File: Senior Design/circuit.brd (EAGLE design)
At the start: 52 x 84.8 mm, 25 parts, among them IC1 74HC164N, IC2 ATMEGA328P, IC3 ATTINY24A, Q1 16 MHz

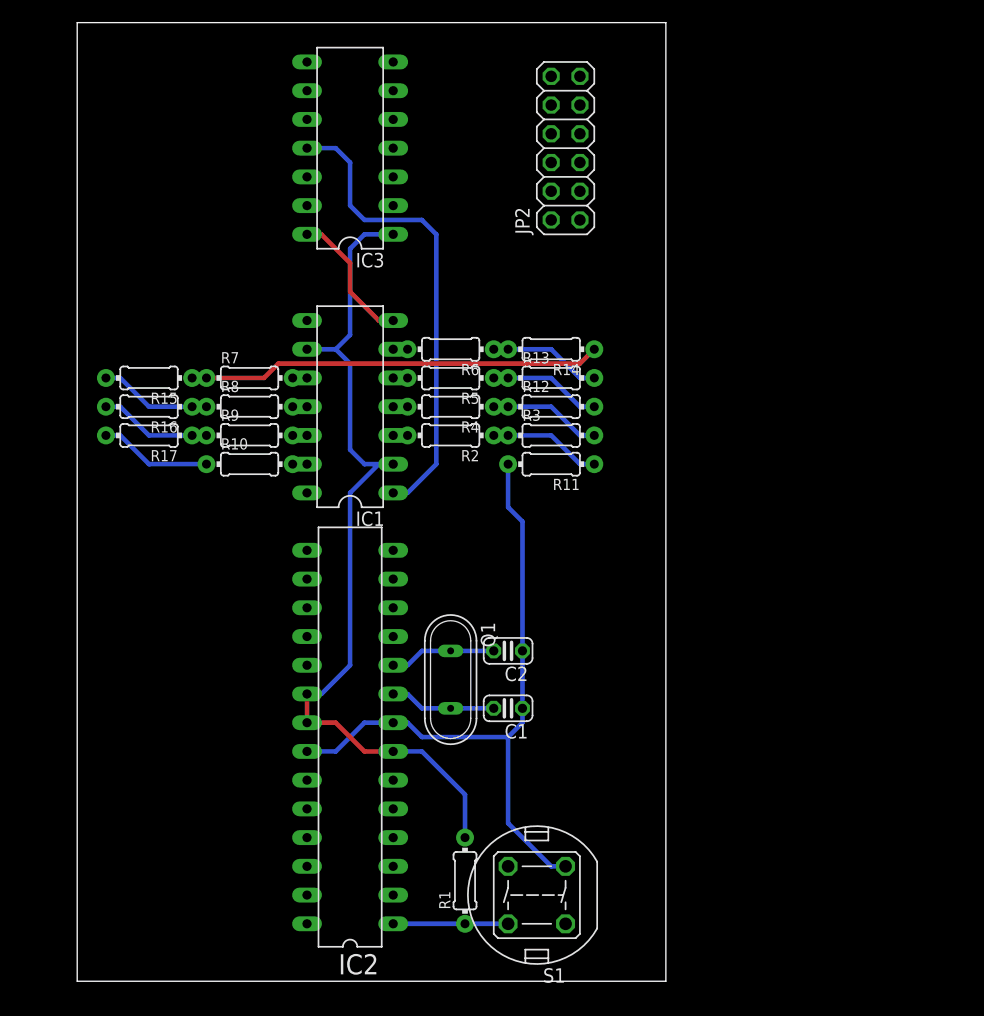
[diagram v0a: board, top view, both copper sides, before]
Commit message: working on senior design circuit and pcb
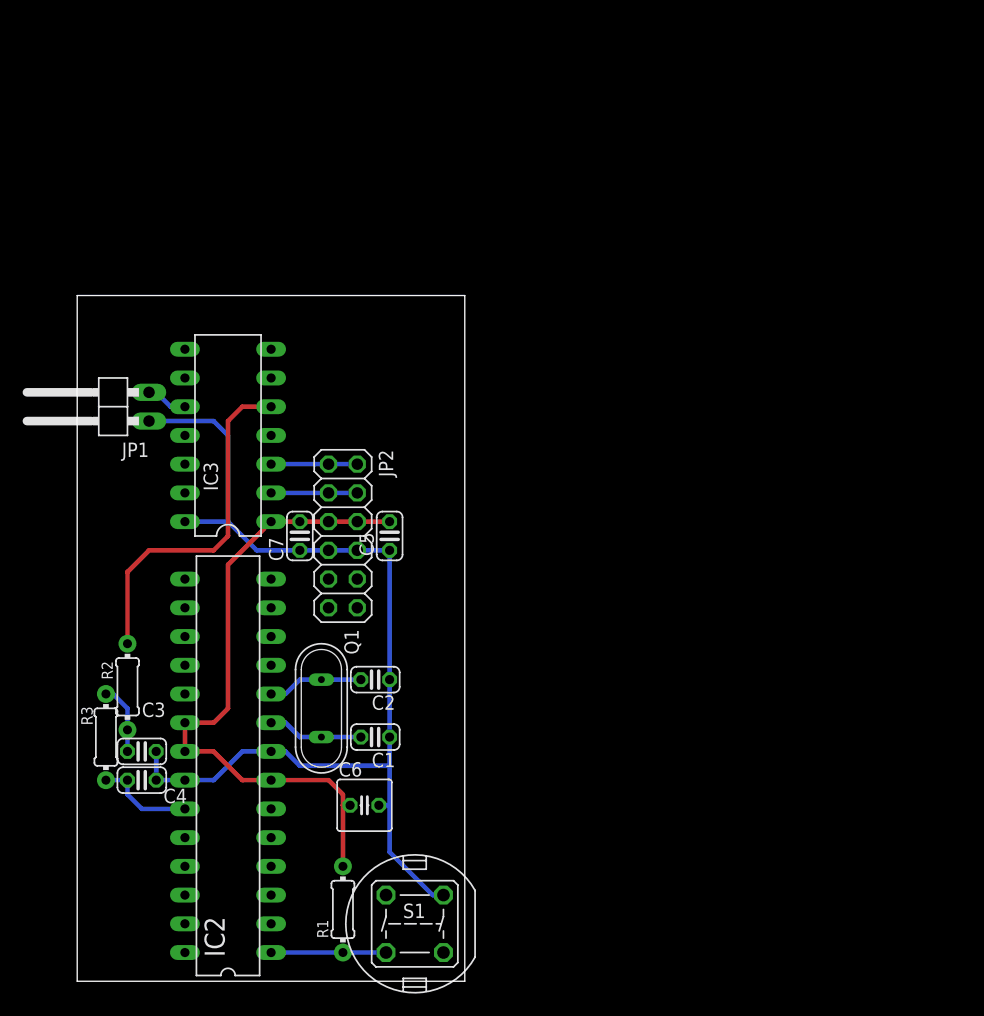
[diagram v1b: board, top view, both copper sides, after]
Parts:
- removed IC1: 74HC164N, 74xx-us:DIL14
- removed R10, R11, R4, R5, R6, R7, R8, R9: 10 kΩ, resistor:0204/7
- removed R12, R13, R14, R15, R16, R17: 4.7 kΩ, resistor:0204/7
- added C3, C4, C5, C7: 10nf, rcl:C025-024X044
- added C6: 100uF, rcl:C025-050X050
- added JP1: (no value), pinhead:1X02/90
- Q1: value 16 MHz -> 16MHz
- R3: value 4.7 kΩ -> 10 kΩ
- moved R3 47.6 mm to (2.54, 21.6), turned to 90 degrees
- moved JP2 39.5 mm to (23.5, 39.4), turned to 270 degrees
- moved R2 36.2 mm to (4.45, 26.0), turned to 90 degrees
- moved IC3 27.6 mm to (12.1, 41.9)
- moved C1 12.0 mm to (26.4, 21.6)
- moved C2 12.0 mm to (26.4, 26.7)
- moved Q1 11.7 mm to (21.6, 24.1)
- moved S1 11.1 mm to (29.8, 5.08)
- moved IC2 11.1 mm to (13.3, 19.1)
- moved R1 11.1 mm to (23.5, 6.35)
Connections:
- removed net N$10: R11.1, R2.1, R3.1
- removed net N$11: R14.1, R15.1, R7.1
- removed net N$12: R15.2, R16.1, R8.1
- removed net N$13: R16.2, R17.1, R9.1
- removed net N$14: R12.2, R13.1, R5.1
- removed net N$15: R12.1, R3.2, R4.1
- removed net N$17: R10.1, R17.2
- removed net N$19: IC1.11, R8.2
- removed net N$25: IC1.4, R4.2
- removed net N$26: IC1.5, R5.2
- removed net N$27: IC1.6, R6.2
- removed net N$28: IC1.10, R7.2
- removed net N$30: IC1.12, R9.2
- removed net N$31: IC1.13, R10.2
- removed net VCC: IC1.14
- net +5V: now also C5.2, C6.1, C7.2, JP2.5, JP2.6; no longer IC1.2, IC1.9, JP2.1, JP2.3
- net GND: now also C3.1, C4.1, C5.1, C6.2, C7.1, JP1.1, JP2.8; no longer IC1.7, JP2.5, R11.2, S1.3
- net N$1: now also IC3.2, JP2.3; no longer IC3.3
- net N$2: now also IC3.3, JP2.1; no longer IC3.2
- net N$3: now also IC3.10, JP1.2; no longer IC1.8, IC3.12
- net N$4: now also IC3.5, R2.2; no longer IC1.1, IC3.11
- net N$7: now also C3.2, R2.1, R3.2; no longer R13.2, R14.2, R6.1
- net N$8: no longer S1.1
- net N$9: now also C4.2, IC2.23, R3.1; no longer IC1.3, R2.2
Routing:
- net N$11: track 36.6 -> 0.00 mm
- net GND: track 71.1 -> 93.0 mm
- net +5V: track 76.7 -> 58.0 mm
- net N$4: track 42.0 -> 31.1 mm
- net N$14: track 9.94 -> 0.00 mm
- net N$12: track 9.94 -> 0.00 mm
- net N$17: track 9.94 -> 0.00 mm
- net N$15: track 9.94 -> 0.00 mm
- net N$13: track 9.94 -> 0.00 mm
- net N$10: track 9.94 -> 0.00 mm
- net N$2: track 0.00 -> 7.62 mm
- net N$1: track 0.00 -> 7.62 mm
- net N$9: track 1.27 -> 8.78 mm
- net N$7: track 11.2 -> 6.24 mm
- net N$3: track 0.00 -> 3.70 mm
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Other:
- board size 52 x 84.8 mm -> 34.3 x 60.6 mm

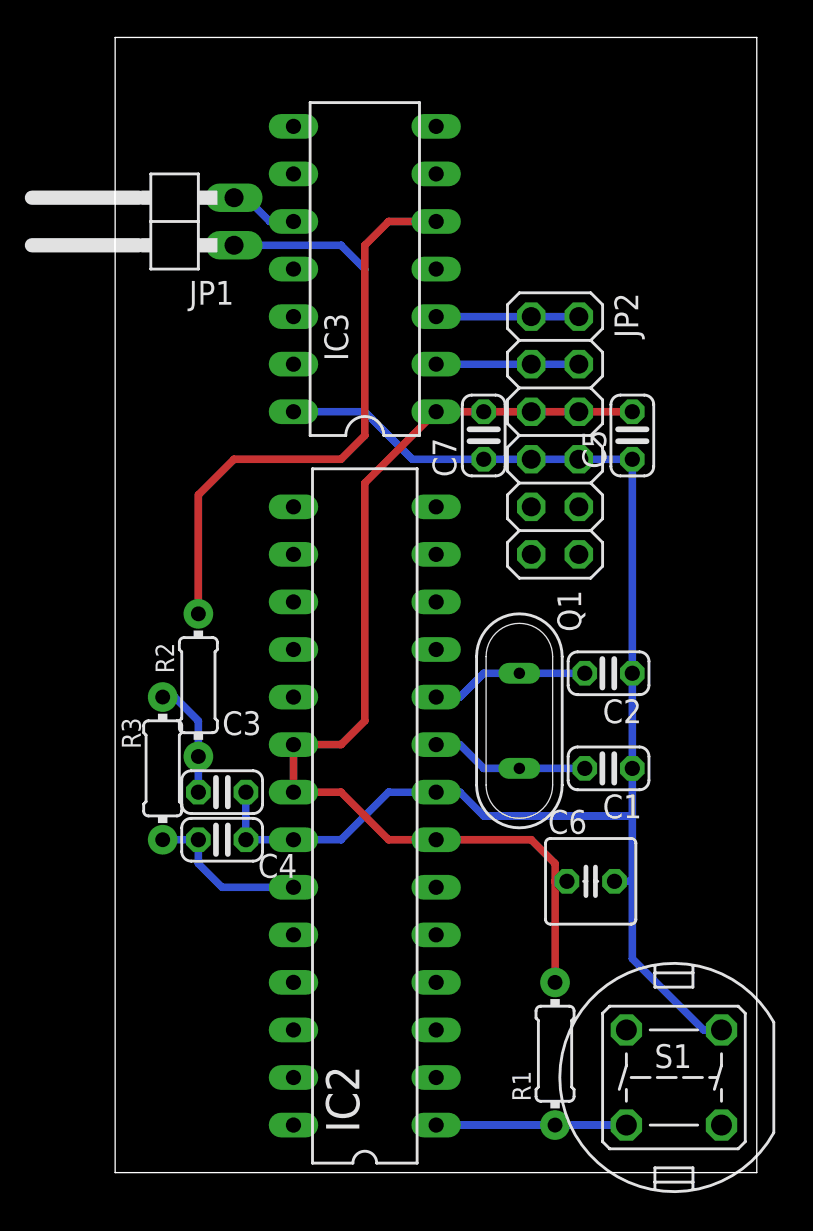
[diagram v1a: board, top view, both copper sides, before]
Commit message: worked on the schematic
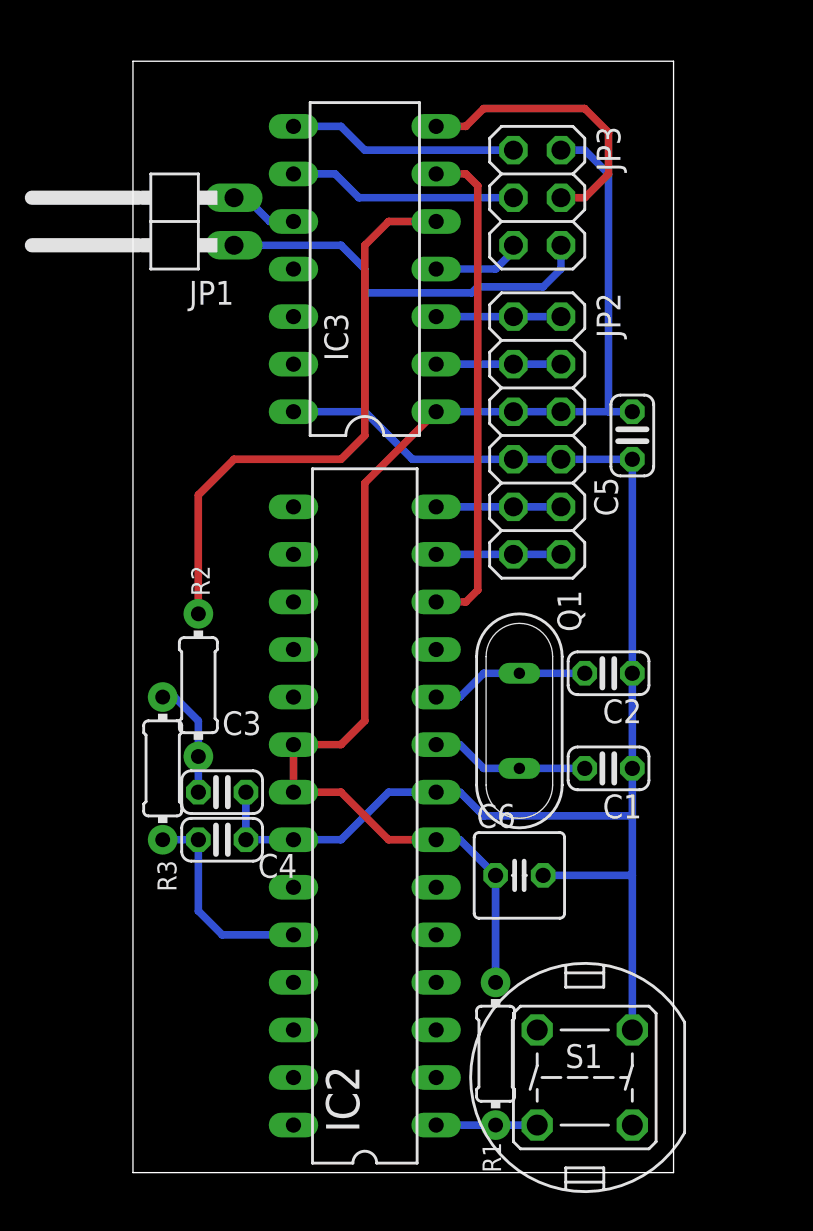
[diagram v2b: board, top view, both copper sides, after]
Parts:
- removed C7: 10nf, rcl:C025-024X044
- added JP3: (no value), pinhead:2X03
- moved S1 4.76 mm to (25.1, 5.08)
- moved C6 3.82 mm to (21.6, 15.9)
- moved R1 3.18 mm to (20.3, 6.35)
- moved JP2 0.95 mm to (22.5, 39.4)
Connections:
- net N$1 renamed P_BSI_DATA
- net N$2 renamed P_SWEEP
- removed net N$9: C4.2, IC2.23, R3.1
- new net DATA-READY: IC2.12, IC3.6
- new net LINE-POSITION: C4.2, IC2.24, R3.1
- new net MISO: IC3.8, JP3.1
- new net MOSI: IC3.7, JP3.4
- new net P_MOTOR: IC2.13, JP2.11, JP2.12
- new net P_STEER: IC2.14, JP2.10, JP2.9
- new net RST: IC3.4, JP3.5
- new net SCK: IC3.9, JP3.3
- net +5V: now also JP3.2; no longer C7.2
- net GND: now also JP3.6; no longer C7.1
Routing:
- net DATA-READY: track 0.00 -> 26.6 mm
- net MOSI: track 0.00 -> 15.4 mm
- net GND: track 93.0 -> 106.6 mm
- net SCK: track 0.00 -> 12.3 mm
- net MISO: track 0.00 -> 12.3 mm
- net +5V: track 58.0 -> 69.6 mm
- net LINE-POSITION: track 0.00 -> 11.3 mm
- net N$9: track 8.78 -> 0.00 mm
- net P_STEER: track 0.00 -> 6.67 mm
- net P_MOTOR: track 0.00 -> 6.67 mm
- net RST: track 0.00 -> 4.84 mm
- net N$8: track 10.2 -> 5.40 mm
- net P_SWEEP: track 7.62 -> 6.67 mm
- net P_BSI_DATA: track 7.62 -> 6.67 mm
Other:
- board size 34.3 x 60.6 mm -> 28.9 x 59.4 mm

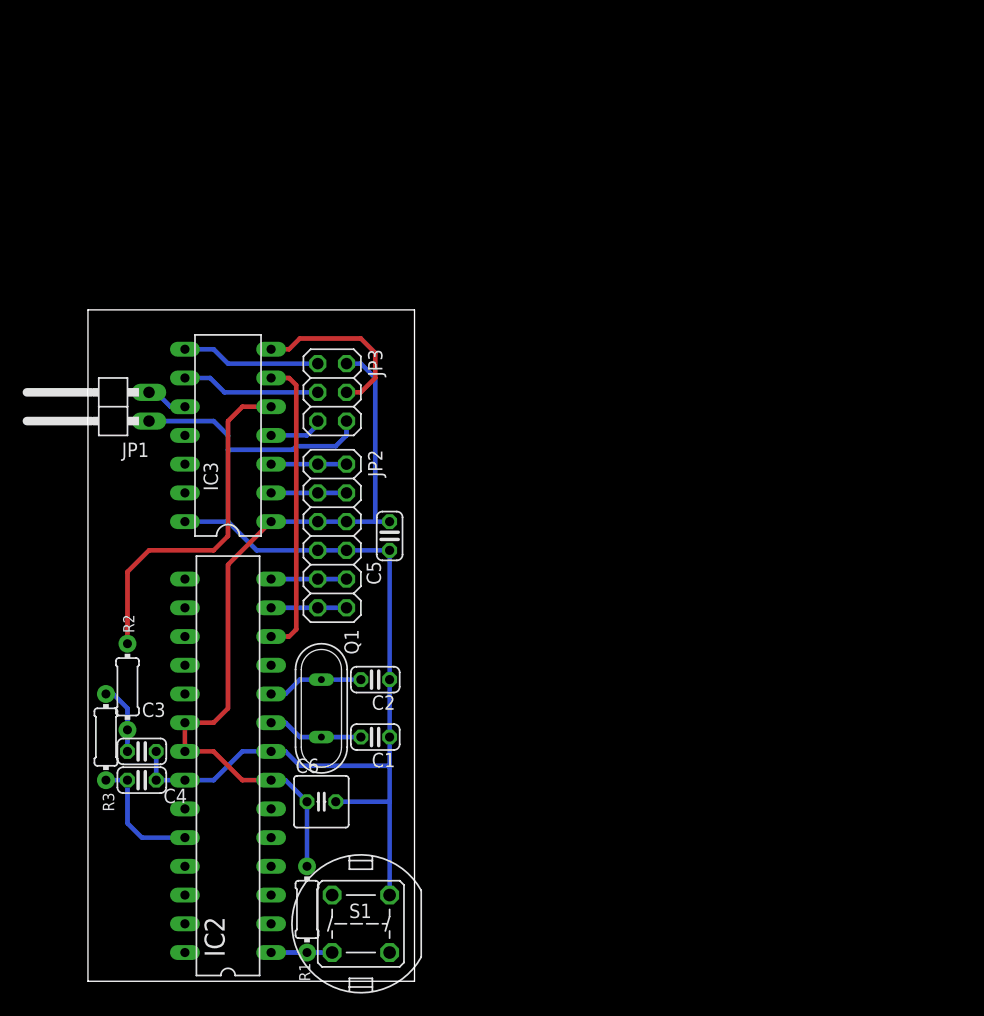
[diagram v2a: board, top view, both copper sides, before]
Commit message: working on senior design and analog switch
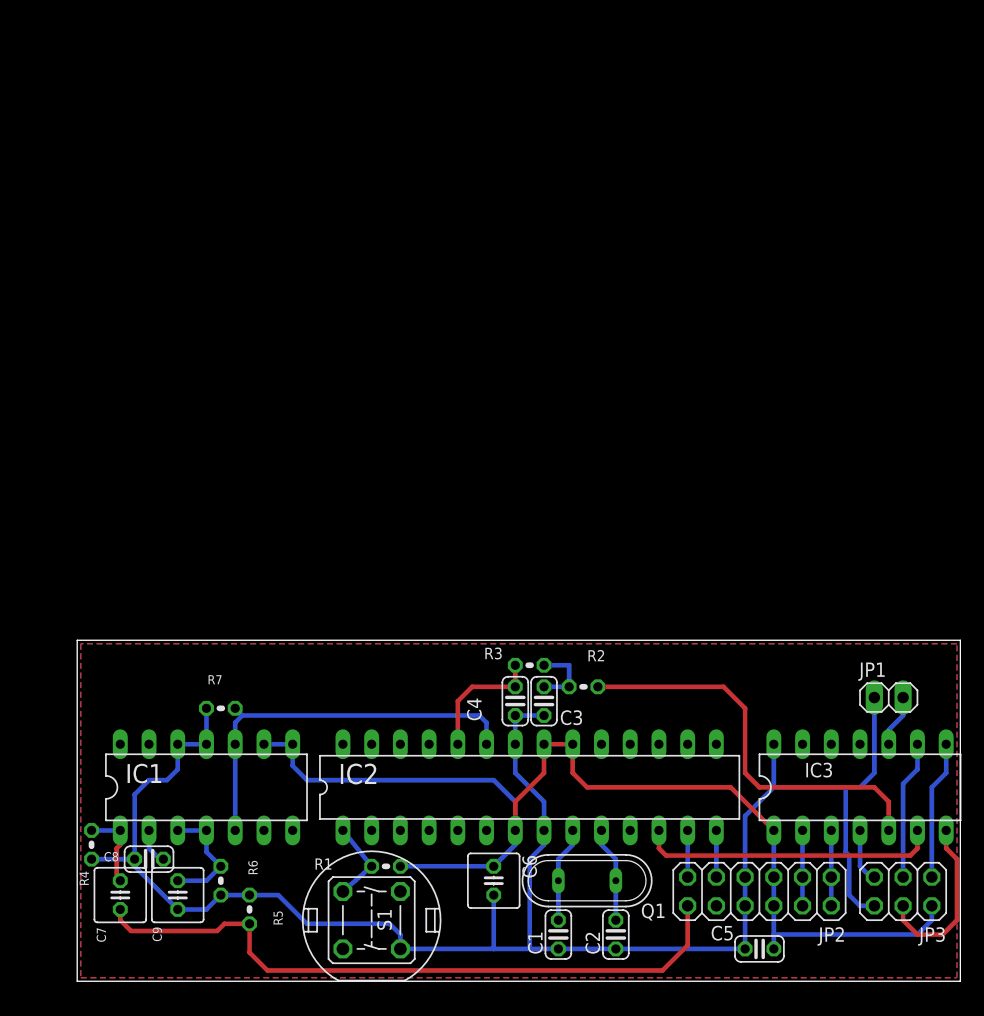
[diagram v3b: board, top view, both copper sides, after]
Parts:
- added C7: 4.7uF, rcl:C025-050X050
- added C8: 10nf, rcl:C025-024X044
- added C9: 1.1uF, rcl:C025-050X050
- added IC1: LM2907, ic-package:DIL14
- added R4: 10 kΩ, resistor:0204V
- added R5: 2.2 kΩ, resistor:0204V
- added R6: 200 kΩ, resistor:0204V
- added R7: 220 kΩ, resistor:0204V
- JP1: device pinhead:1X02/90 -> pinhead:1X02
- R1, R2, R3: device resistor:0204/7 -> resistor:0204V
- moved JP1 73.8 mm to (71.8, 25.1), turned to 0 degrees
- moved JP3 67.1 mm to (73.0, 7.94), turned to 180 degrees
- moved IC3 56.0 mm to (62.9, 18.4), turned to 0 degrees
- moved JP2 49.1 mm to (60.3, 7.94), turned to 180 degrees
- moved C5 49.0 mm to (60.3, 2.86), turned to 0 degrees
- moved R2 40.3 mm to (44.8, 26.0), turned to 0 degrees
- moved R3 38.0 mm to (40.0, 27.9), turned to 0 degrees
- moved C3 35.8 mm to (41.3, 24.8), turned to 90 degrees
- moved C4 33.8 mm to (38.7, 24.8), turned to 90 degrees
- moved C2 31.0 mm to (47.6, 4.13), turned to 90 degrees
- moved Q1 28.0 mm to (45.1, 8.89), turned to 180 degrees
- moved IC2 26.7 mm to (40.0, 17.1), turned to 0 degrees
- moved C1 23.8 mm to (42.5, 4.13), turned to 90 degrees
- moved C6 16.8 mm to (36.8, 8.89), turned to 270 degrees
- moved R1 7.96 mm to (27.3, 10.2), turned to 0 degrees
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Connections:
- new net FIN: C7.1, JP2.12, R5.2
- new net N$1: C9.1, IC1.3, IC1.4, R6.1
- new net N$12: C8.2, IC1.2
- new net N$9: C7.2, IC1.1, R4.1
- new net V_FREQ: IC1.10, IC1.5, IC2.23, R7.2
- net +5V: now also IC1.8, IC1.9
- net GND: now also C8.1, C9.2, IC1.11, IC1.12, R4.2, R5.1, R6.2, R7.1
- net P_MOTOR: no longer JP2.12
- net P_STEER: no longer JP2.10
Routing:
- net FIN: track 0.00 -> 59.4 mm
- net GND: track 106.6 -> 158.6 mm
- net V_FREQ: track 0.00 -> 35.1 mm
- net +5V: track 69.6 -> 100.1 mm
- net N$1: track 0.00 -> 10.6 mm
- net N$9: track 0.00 -> 7.25 mm
- net N$4: track 31.1 -> 35.8 mm
- net N$12: track 0.00 -> 3.25 mm
- net P_STEER: track 6.67 -> 4.13 mm
- net P_MOTOR: track 6.67 -> 4.13 mm
- net N$8: track 5.40 -> 7.44 mm
- net N$3: track 3.70 -> 4.65 mm
- added copper zone on layer 1, net GND
- added copper zone on layer 16, net GND
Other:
- board size 28.9 x 59.4 mm -> 78.1 x 30.1 mm
